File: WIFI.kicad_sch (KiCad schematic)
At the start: 34 parts, among them J3 ESP Anten, SW2 ESP_RESET, SW3 ESP_BOOT, U4 ESP32-D0WD-V3, U5 W25Q32JVSS, Y3 40MHz

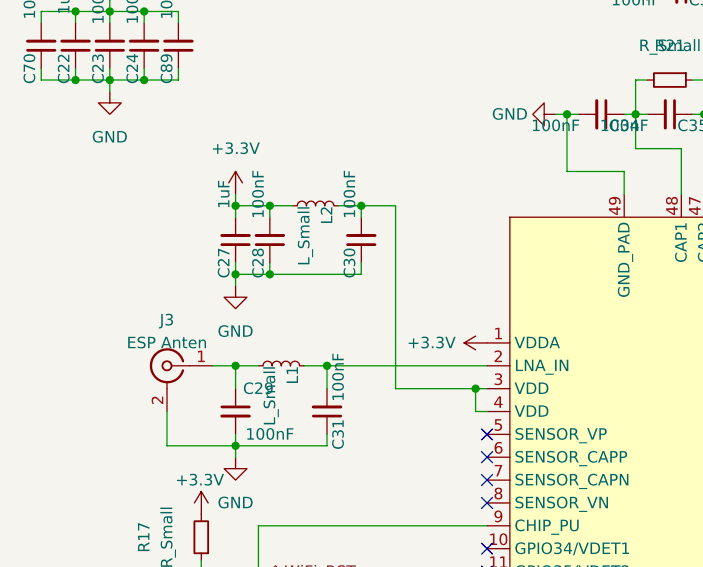
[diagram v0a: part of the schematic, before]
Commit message: Only 1 wire to complete.
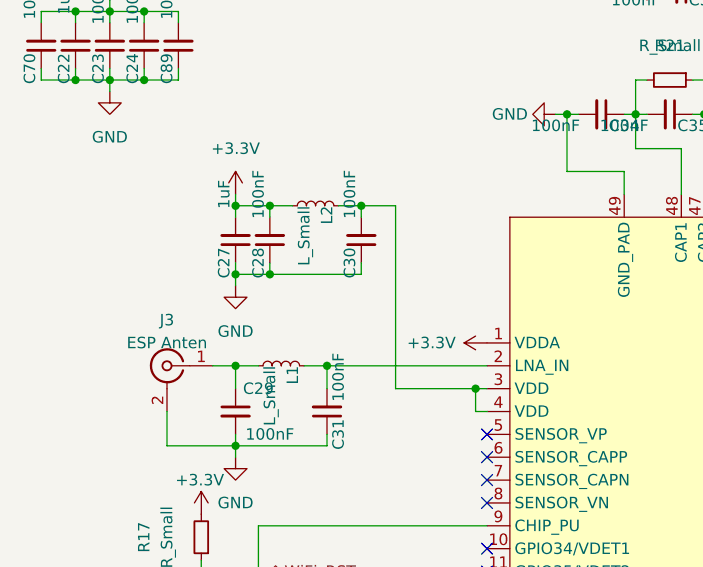
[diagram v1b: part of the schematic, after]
